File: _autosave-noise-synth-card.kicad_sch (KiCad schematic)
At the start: 43 parts, among them J1 CVpitch, J2 FM in, J3 PWM in, M1 imogen-wren-card, Q1 BC558, Q2 BC548, U1 TL074, U2 TL074, U3 HEF4093B

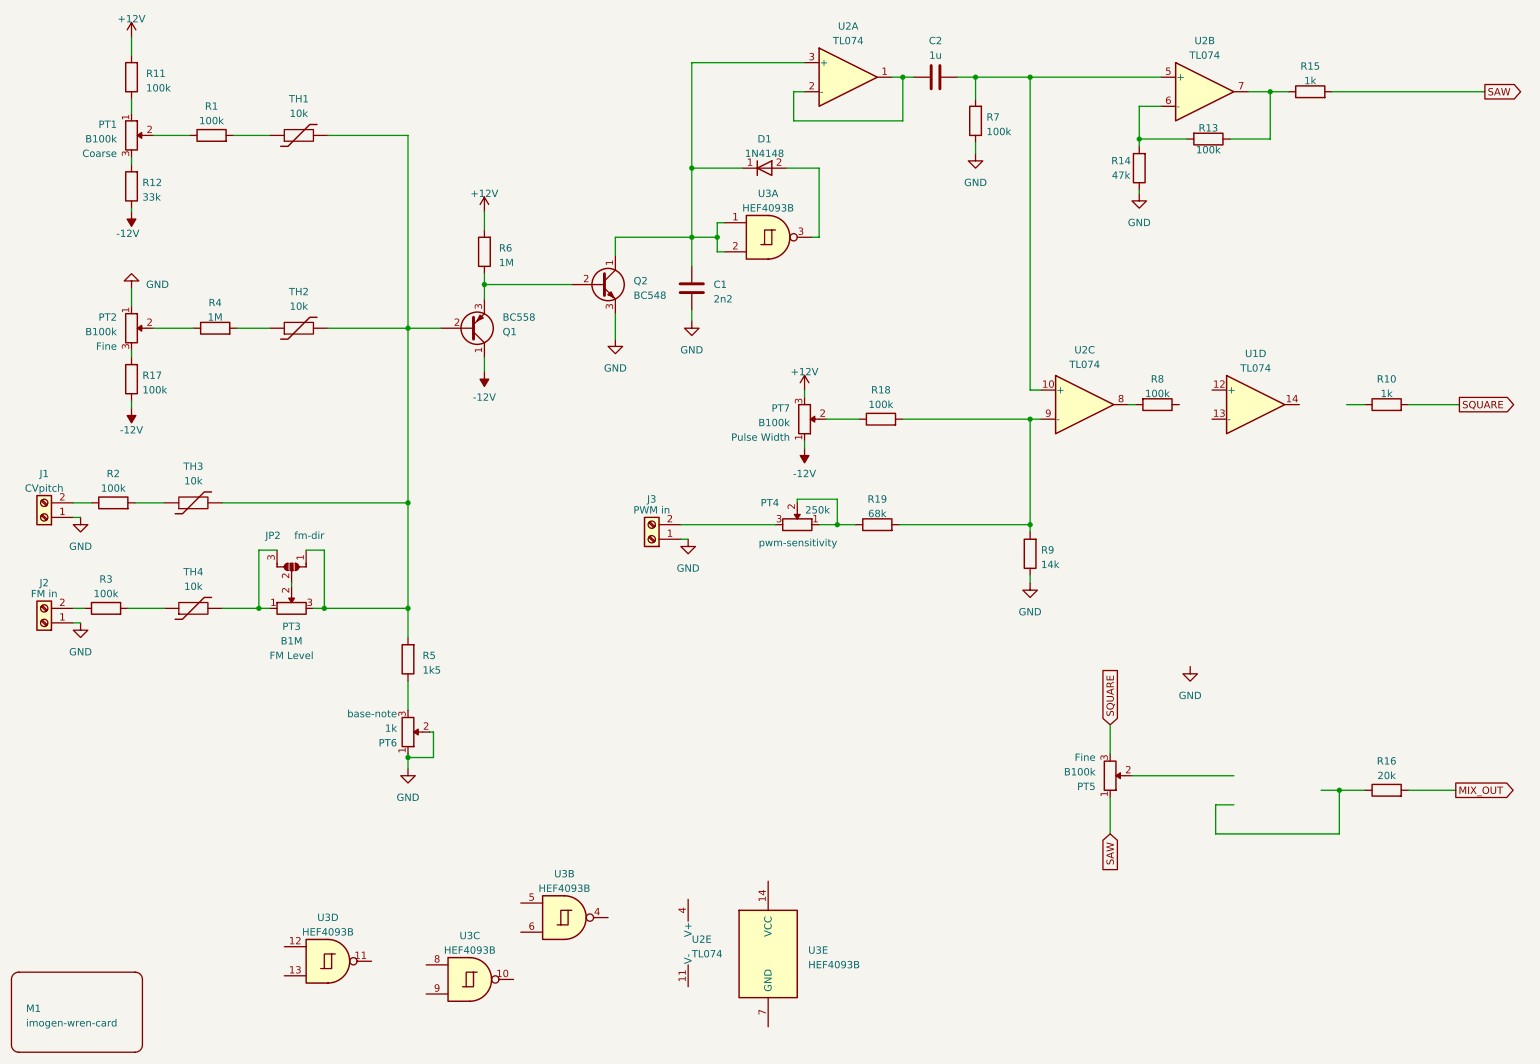
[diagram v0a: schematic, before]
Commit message: fixed shcematic
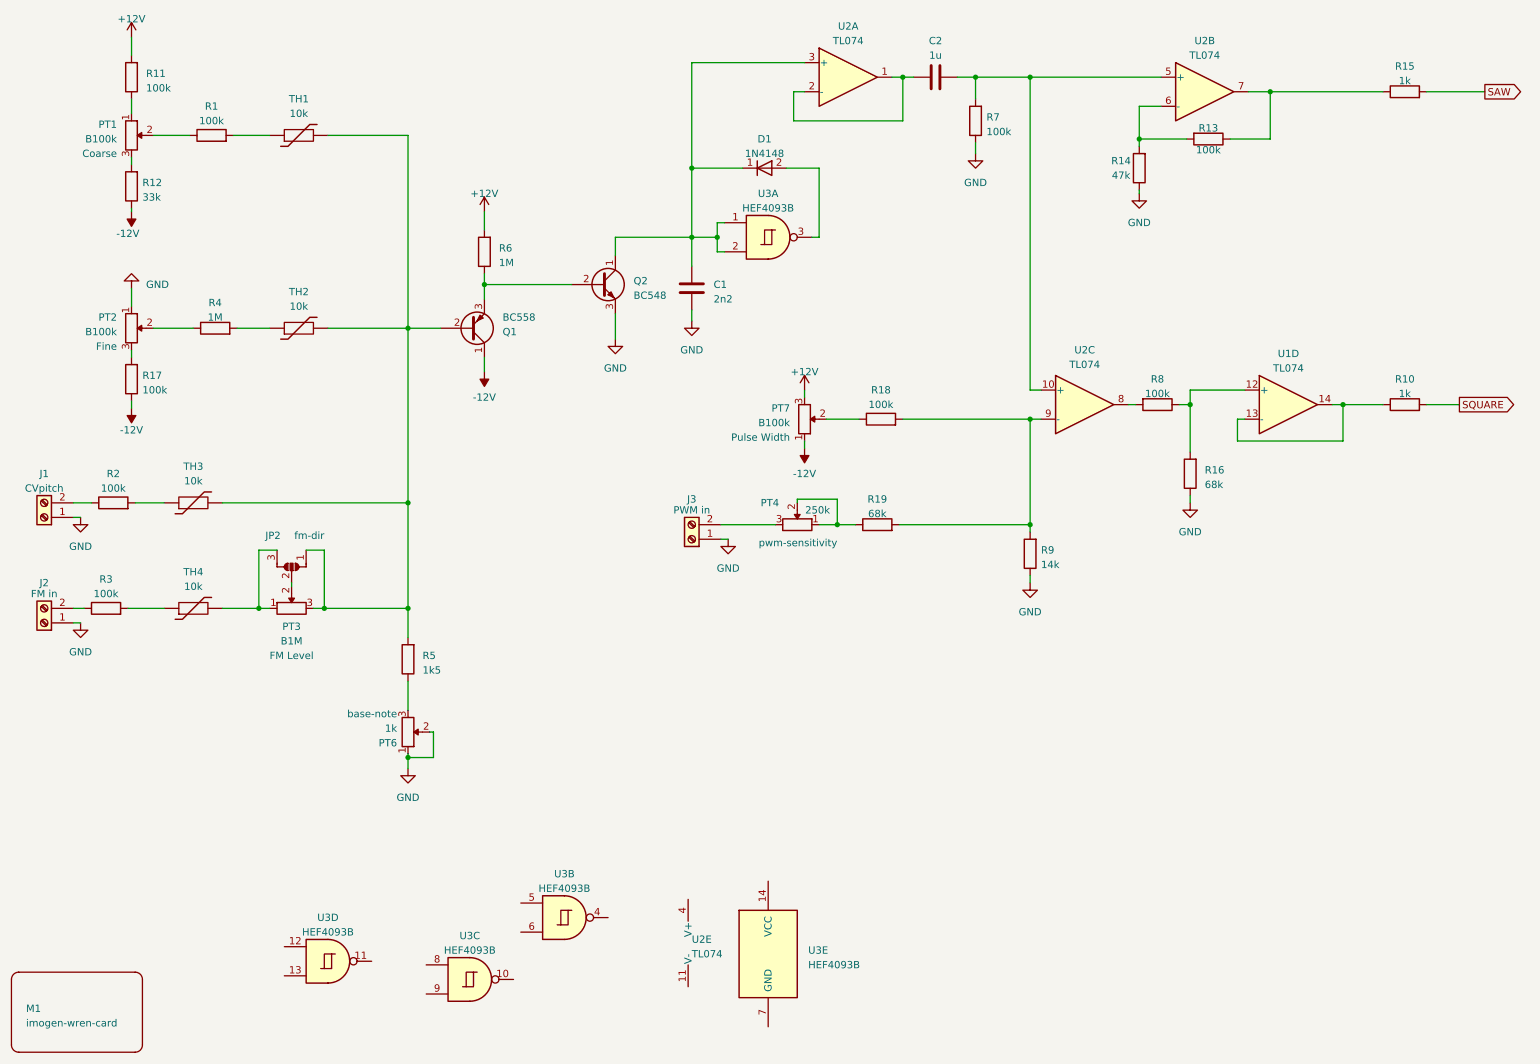
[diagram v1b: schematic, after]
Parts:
- removed PT5: B100k, Potentiometer_THT:Potentiometer_Alpha_RD901F-40-00D_Single_Vertical_CircularHoles, symbol 000_Resistors_Immo:Alpha Pot
- R16: value 20k -> 68k
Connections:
- net MIX_OUT is gone; now on an unnamed net: R16.2
- net GND: now also R16.1
- net at U1.12 (+): now also R8.1
- net at U1.13 (-): now also R10.1, U1.14
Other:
- moved on the sheet: J3, R10, R15, U1D
